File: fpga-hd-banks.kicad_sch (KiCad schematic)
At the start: 16 parts, among them Q4 BSS138PW, Q5 BSS138PW, Q6 BSS138PW, Q7 BSS138PW, Q8 BSS138PW, U34 XCAU25P-2FFVB676I

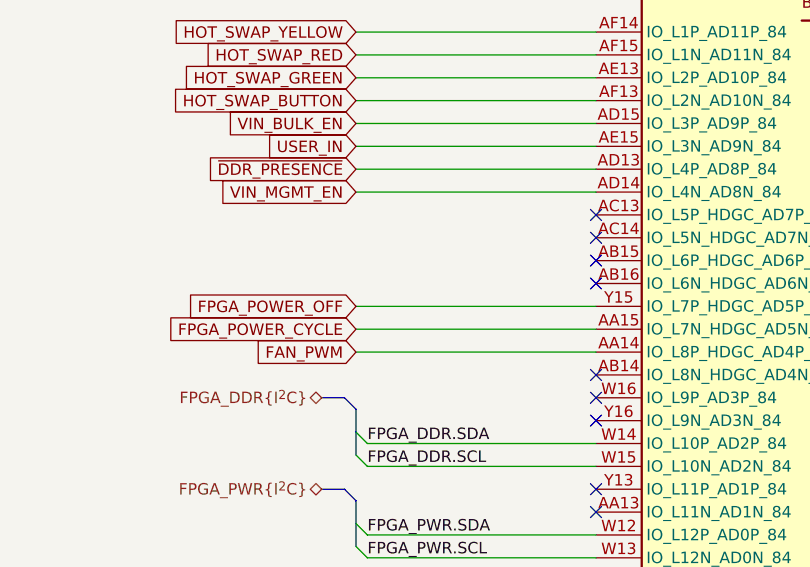
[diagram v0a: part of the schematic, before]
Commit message: [#68088] Add heater connector
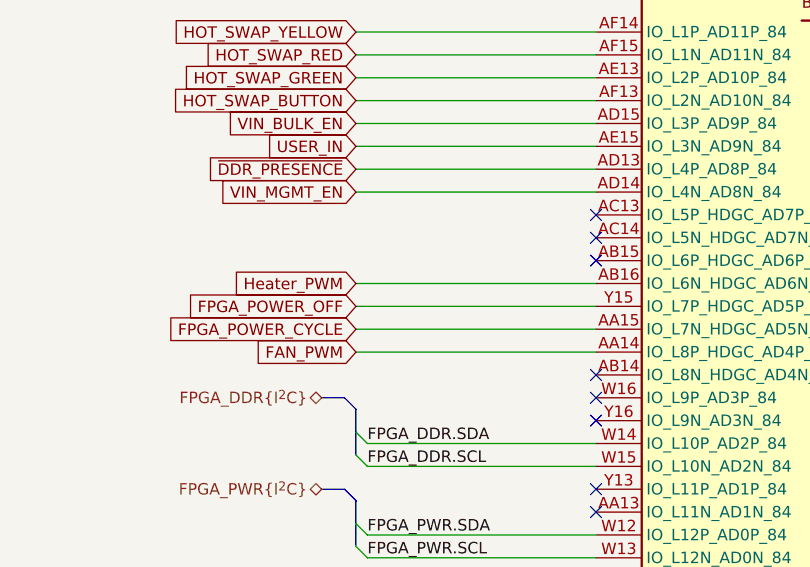
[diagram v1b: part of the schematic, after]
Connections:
- net Heater_PWM: now reaches U34.AB16 (IO_L6N_HDGC_AD6N_84)
- no-connect marks 24 -> 23
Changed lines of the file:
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@@
   (no_connect (at 205.74 92.71))
   (no_connect (at 205.74 95.25))
-  (no_connect (at 318.77 105.41))
   (no_connect (at 318.77 97.79))
   (no_connect (at 93.98 95.25))
@@
     (stroke (width 0) (type default))
   )
+  (wire (pts (xy 292.1 105.41) (xy 318.77 105.41))
+    (stroke (width 0) (type default))
+  )
   (wire (pts (xy 292.1 107.95) (xy 318.77 107.95))
     (stroke (width 0) (type default))
@@
       (effects (font (size 1.27 1.27)) (justify right))
     )
+  )
+  (global_label "Heater_PWM" (shape input) (at 292.1 105.41 180) (fields_autoplaced)
+    (effects (font (size 1.27 1.27)) (justify right))
+    (property "Intersheetrefs" "${INTERSHEET_REFS}" (at 278.46 105.41 0)
+      (effects (font (size 1.27 1.27)) (justify right))
+    )
